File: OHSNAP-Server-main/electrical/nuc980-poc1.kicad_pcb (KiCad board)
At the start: 2 copper layers, 101.6 x 76.2 mm, 110 parts, among them J1 5-6VDC in, J2 JTAG, J3 FTDI, J4 USB-A, J5 Conn_01x08, J6 Molex MicroSD 503182-1852, Q1 MMBT3904, SW1 User Button, SW2 Boot Source, SW3 Reset, U1 PAM2306AYPKE, U2 W25Q128JVS, U3 LM3670MF, U4 NUC980DR61YC, Y1 12 MHz

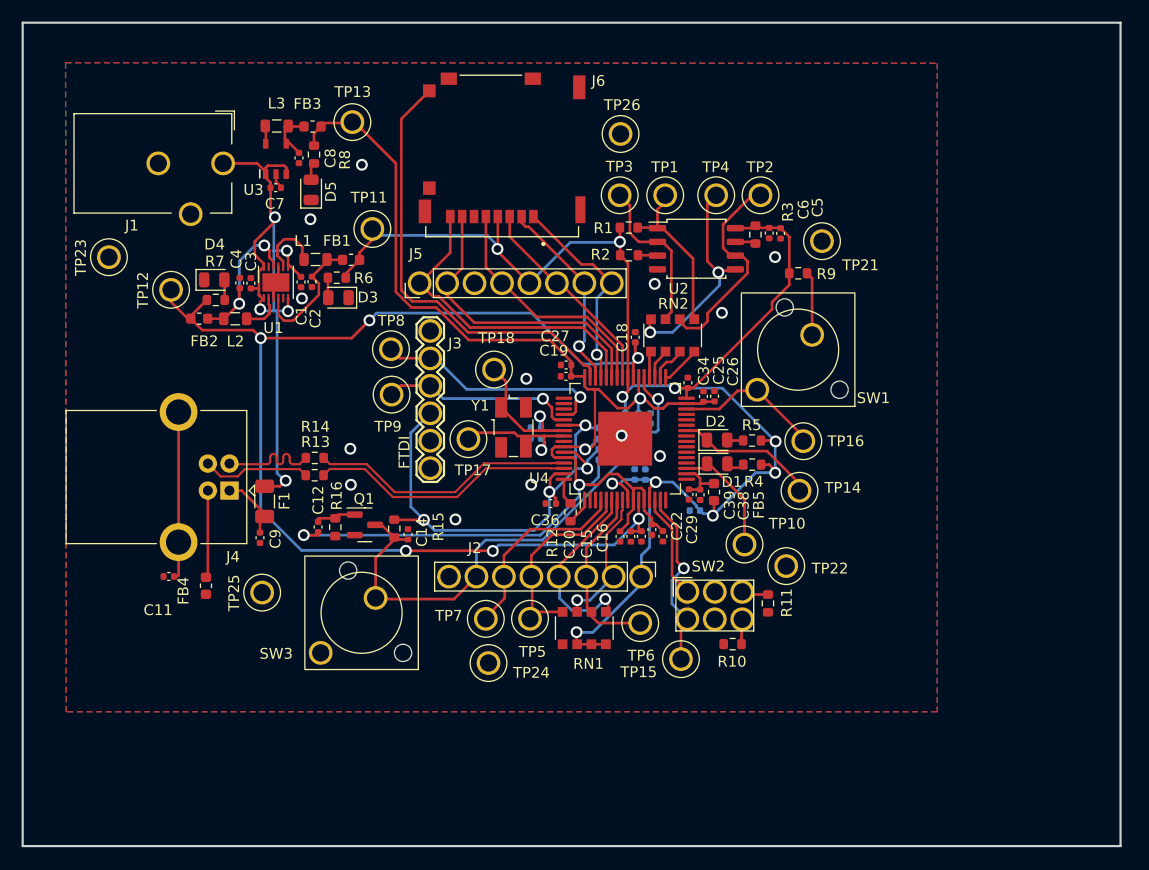
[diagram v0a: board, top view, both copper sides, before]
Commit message: Add files via upload
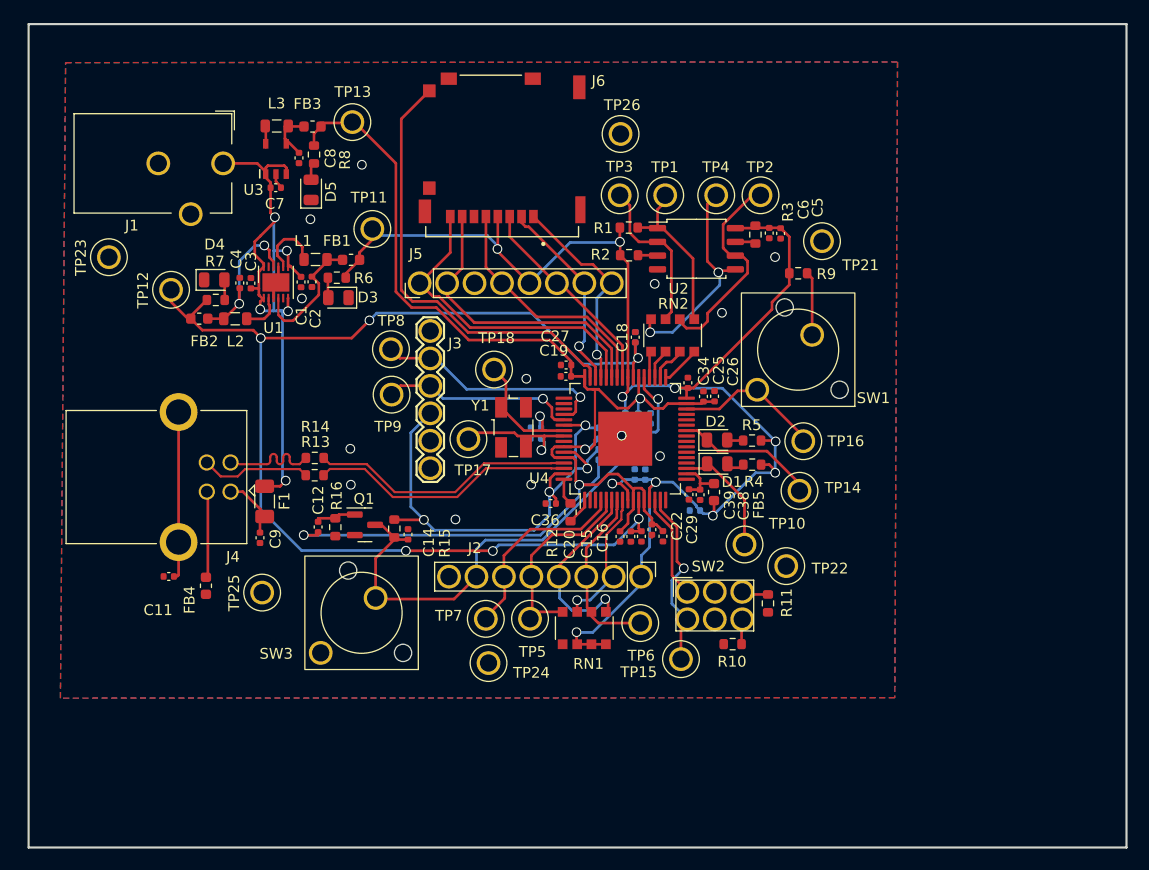
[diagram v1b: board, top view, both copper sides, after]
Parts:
- J3: value FTDI -> Serial FTDI Header
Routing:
- net Net-(J2-Pin_2): track 12.9 -> 13.5 mm
